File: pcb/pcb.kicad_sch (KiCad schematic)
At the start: 76 parts, among them J1 OLED Display, J2 U1_Header_1, J3 U1_Header_2, SW1 SW_SPDT, SW2 SW_Push, SW3 SW_Push, SW4 SW_Push, U1 MOUDLE-SEEEDUINO-XIAO-ESP32S3

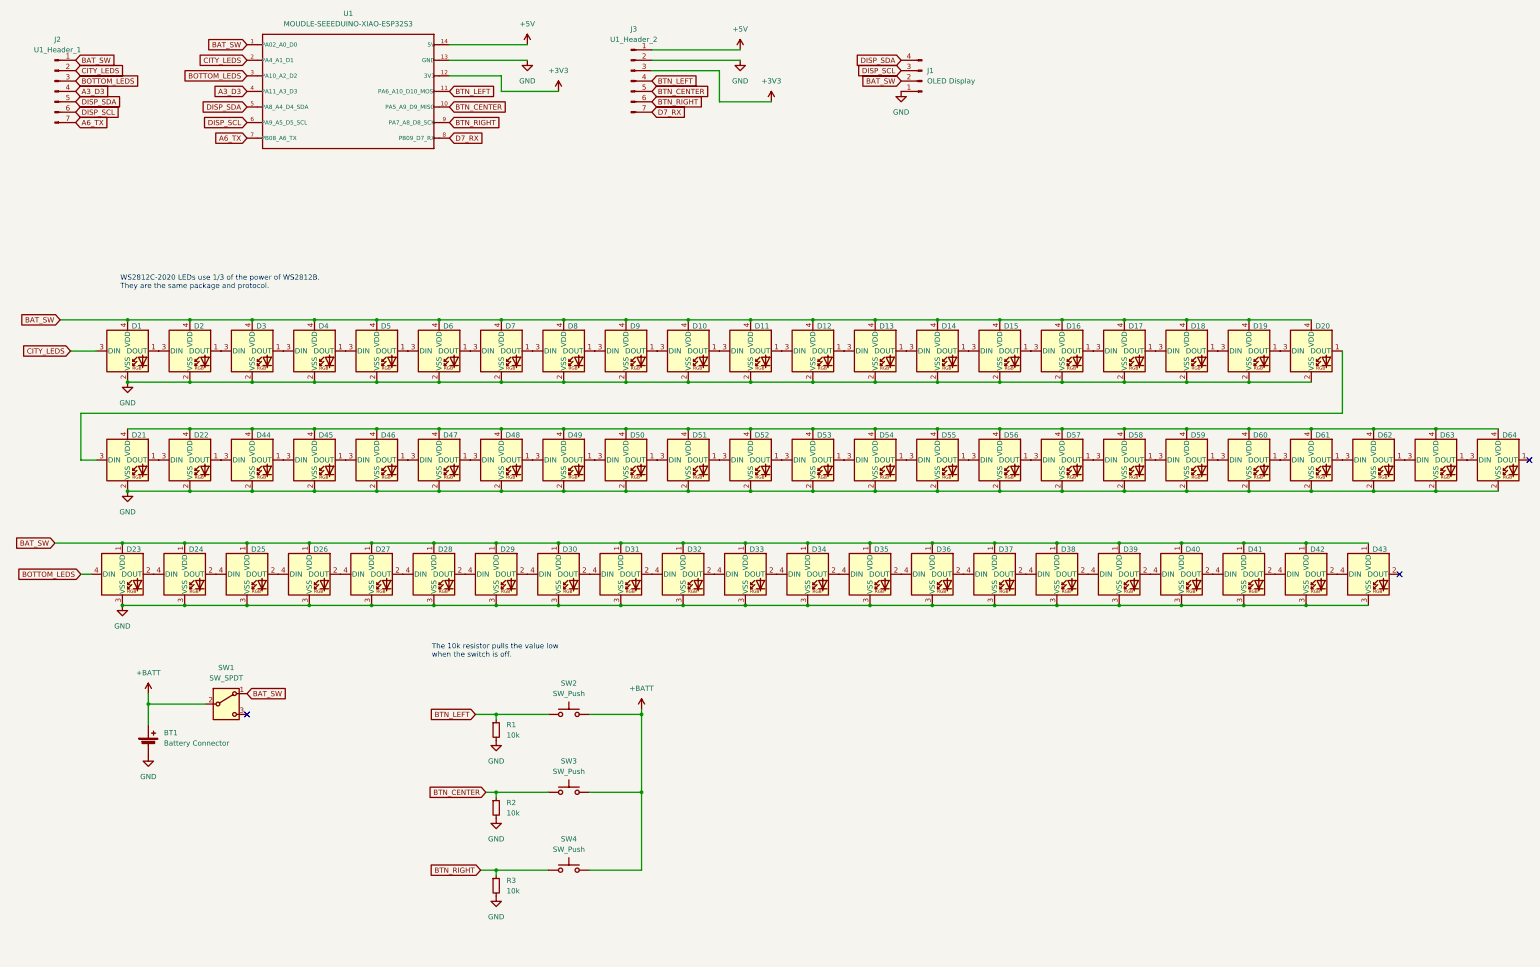
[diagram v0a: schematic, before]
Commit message: Almost there
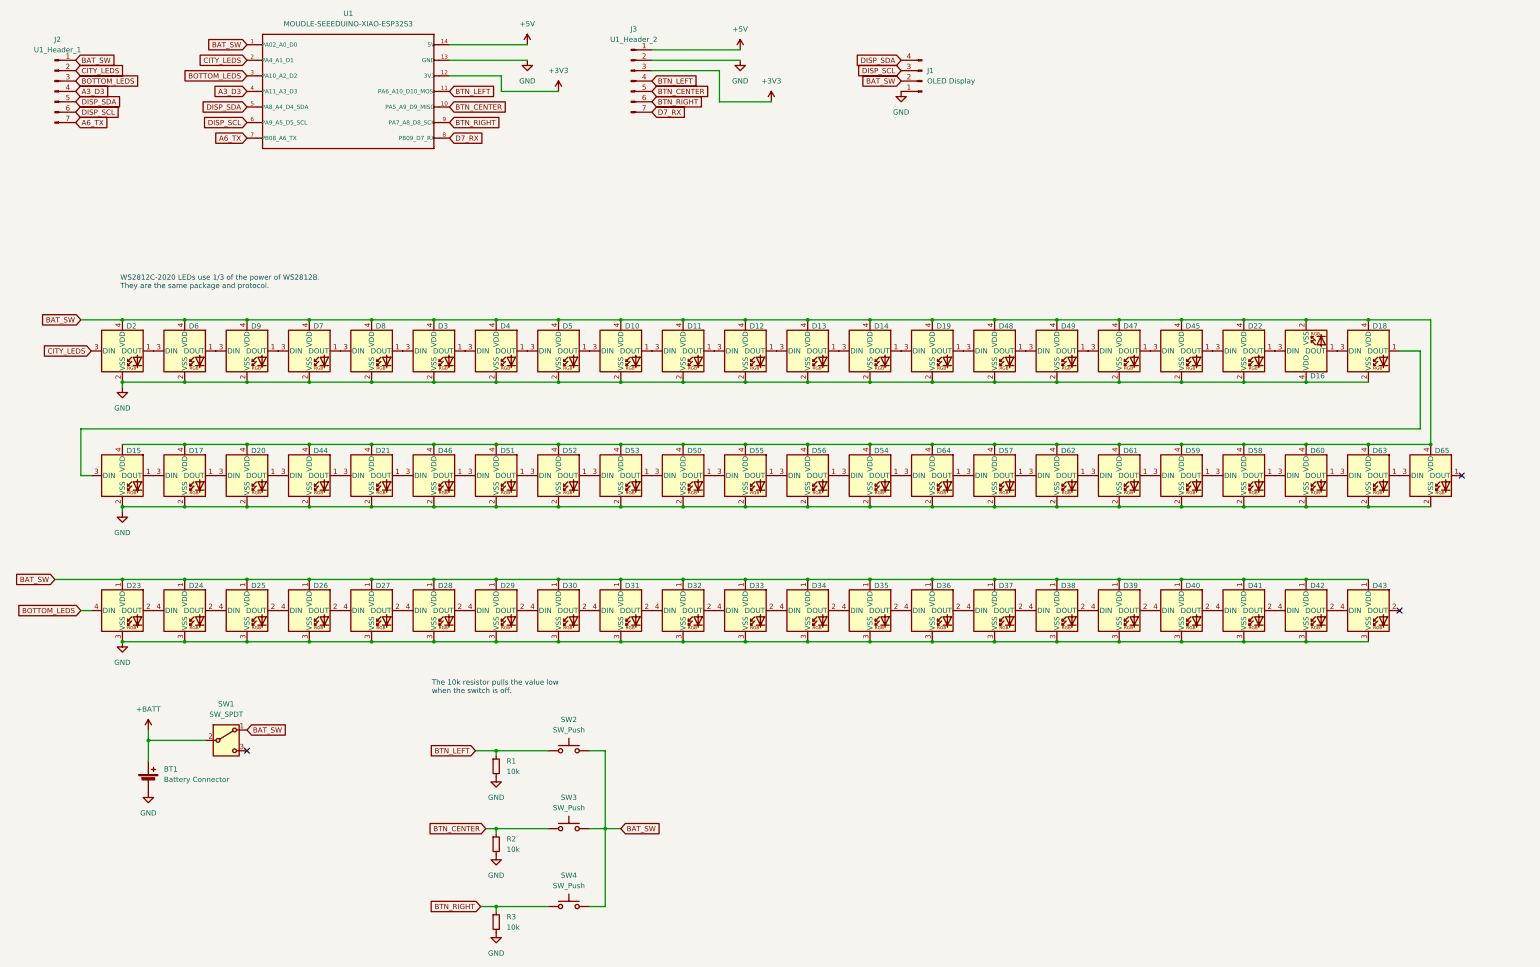
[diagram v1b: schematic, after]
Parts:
- renumbered D1 to D65
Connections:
- net +BATT: no longer SW2.2, SW3.2, SW4.2
- net BAT_SW: now also D16.2 (VSS), D21.4 (VDD), D22.4 (VDD), D44.4 (VDD), D45.4 (VDD), D46.4 (VDD), D47.4 (VDD), D48.4 (VDD), D49.4 (VDD), D50.4 (VDD), D51.4 (VDD), D52.4 (VDD), D53.4 (VDD), D54.4 (VDD), D55.4 (VDD), D56.4 (VDD), D57.4 (VDD), D58.4 (VDD), D59.4 (VDD), D60.4 (VDD), D61.4 (VDD), D62.4 (VDD), D63.4 (VDD), D64.4 (VDD), SW2.2, SW3.2, SW4.2; no longer D16.4 (VDD)
- net CITY_LEDS: now also D2.3 (DIN); no longer D65.3 (DIN)
- net GND: now also D16.4 (VDD); no longer D16.2 (VSS)
- net at D53.1 (DOUT): now also D50.3 (DIN); no longer D54.3 (DIN)
- net at D20.1 (DOUT): now also D44.3 (DIN); no longer D21.3 (DIN)
- net at D20.3 (DIN): now also D17.1 (DOUT); no longer D19.1 (DOUT)
- net at D10.3 (DIN): now also D5.1 (DOUT); no longer D9.1 (DOUT)
- net at D9.3 (DIN): now also D6.1 (DOUT); no longer D8.1 (DOUT)
- net at D49.1 (DOUT): now also D47.3 (DIN); no longer D50.3 (DIN)
- net at D22.1 (DOUT): now also D16.3 (DIN); no longer D44.3 (DIN)
- net at D22.3 (DIN): now also D45.1 (DOUT); no longer D21.1 (DOUT)
- net at D57.1 (DOUT): now also D62.3 (DIN); no longer D58.3 (DIN)
- net at D57.3 (DIN): now also D64.1 (DOUT); no longer D56.1 (DOUT)
- net at D19.3 (DIN): now also D14.1 (DOUT); no longer D18.1 (DOUT)
- net at D18.3 (DIN): now also D16.1 (DOUT); no longer D17.1 (DOUT)
- net at D17.3 (DIN): now also D15.1 (DOUT); no longer D16.1 (DOUT)
- net at D59.1 (DOUT): now also D58.3 (DIN); no longer D60.3 (DIN)
- net at D59.3 (DIN): now also D61.1 (DOUT); no longer D58.1 (DOUT)
- net at D46.3 (DIN): now also D21.1 (DOUT); no longer D45.1 (DOUT)
- net at D45.3 (DIN): now also D47.1 (DOUT); no longer D44.1 (DOUT)
- net at D7.3 (DIN): now also D9.1 (DOUT); no longer D6.1 (DOUT)
- net at D6.3 (DIN): now also D2.1 (DOUT); no longer D5.1 (DOUT)
- net at D61.3 (DIN): now also D62.1 (DOUT); no longer D60.1 (DOUT)
- net at D46.1 (DOUT): now also D51.3 (DIN); no longer D47.3 (DIN)
- net at D63.3 (DIN): now also D60.1 (DOUT); no longer D62.1 (DOUT)
- net at D50.1 (DOUT): now also D55.3 (DIN); no longer D51.3 (DIN)
- net at D54.1 (DOUT): now also D64.3 (DIN); no longer D55.3 (DIN)
- net at D63.1 (DOUT): now also D65.3 (DIN); no longer D64.3 (DIN)
- net at D3.3 (DIN): now also D8.1 (DOUT); no longer D2.1 (DOUT)
- net at D65.1 (DOUT): no longer D2.3 (DIN)
- net at D48.3 (DIN): now also D19.1 (DOUT); no longer D47.1 (DOUT)
- net at D15.3 (DIN): now also D18.1 (DOUT); no longer D14.1 (DOUT)
- new net: D54.3 (DIN), D56.1 (DOUT)
- new net: D58.1 (DOUT), D60.3 (DIN)
- new net: D21.3 (DIN), D44.1 (DOUT)
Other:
- moved on the sheet: BT1, D10, D11, D12, D13, D14, D15, D16, D17, D18, D19, D2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
